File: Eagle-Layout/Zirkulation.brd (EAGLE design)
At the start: 50 x 50 mm, 13 parts, among them X1 MKDSN1,5/3-5,08

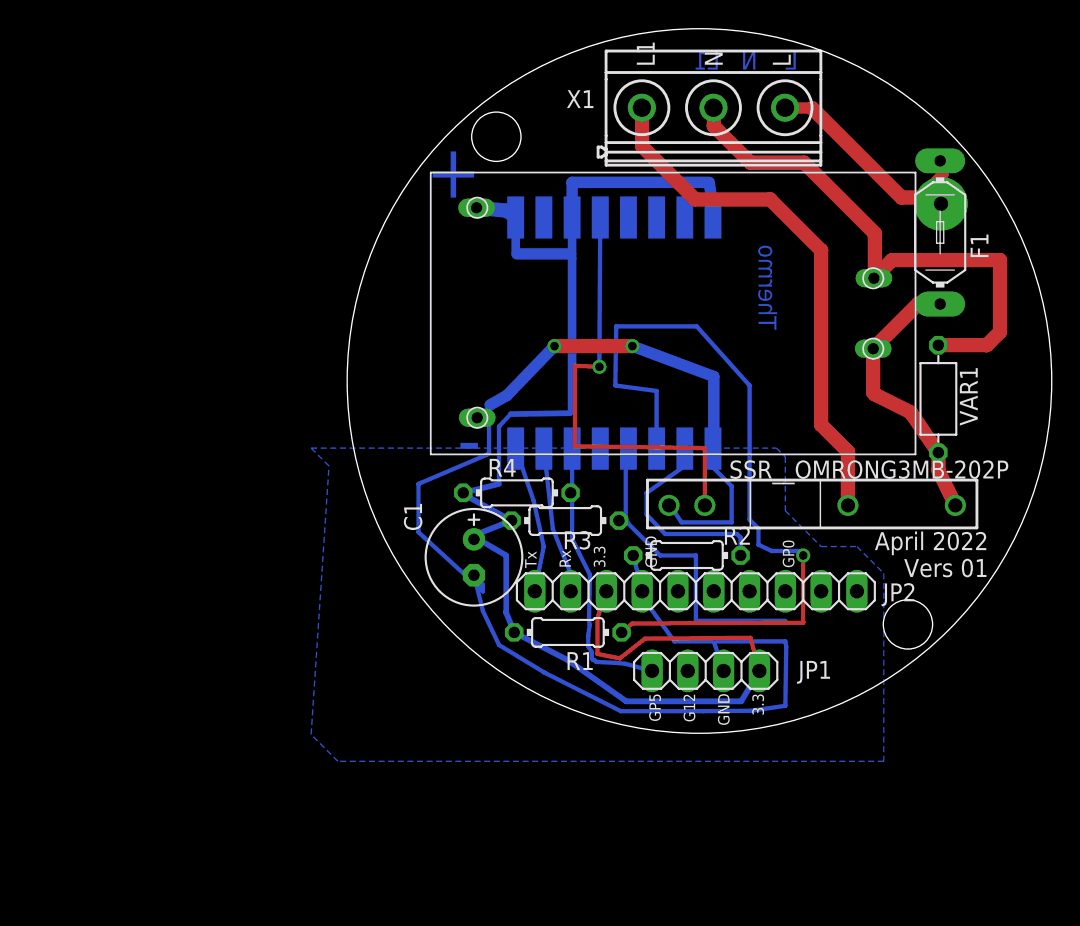
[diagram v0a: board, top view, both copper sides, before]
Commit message: Personal custom variant of Heise Zirkulationspumpe
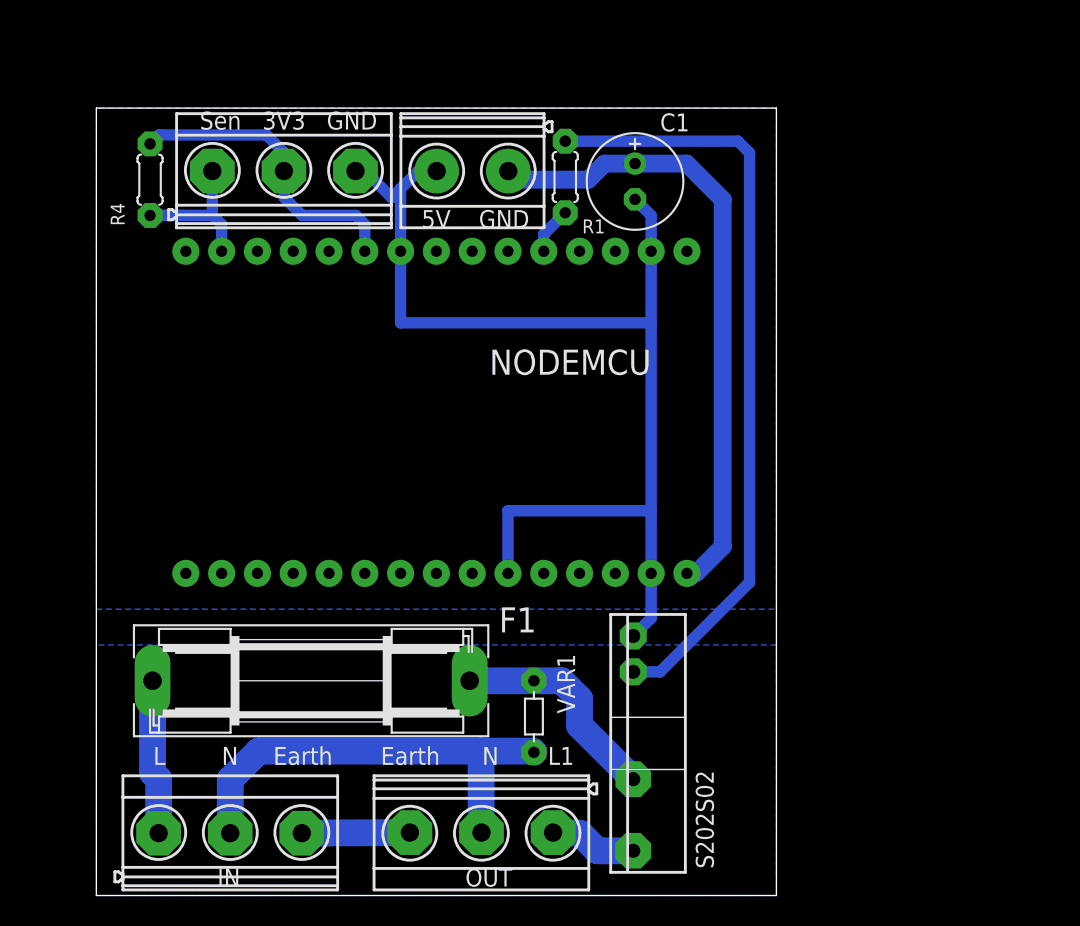
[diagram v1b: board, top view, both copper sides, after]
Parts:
- removed ESP-12E/F: ESP8266, esp8266modules:ESP12-SMD
- removed JP1: Temp.Sensor 18B20, pinhead:1X04
- removed JP2: Prog-Schnittstelle, pinhead:1X10
- removed PRINTTRAFO3.3V,_3W: PRINTTRAFO, Uwes_lib:PRINTTRAFO
- removed R2: 2,2K, rcl:0204/7
- removed R3: 10K, rcl:0204/7
- removed SSR__OMRONG3MB-202P: S102S02, relay:S202S02
- removed X1: MKDSN1,5/3-5,08, con-phoenix-508:MKDSN1,5/3-5,08
- added IN, OUT, SENSOR: MKDSN1,5/3-5,08, my_con-phoenix-508:MKDSN1,5/3-5,08
- added NODEMCU: ESP12E_DEVKIT, ESP12E_DEVKIT:ESP12E_DEVKIT
- added PWR: MKDSN1,5/2-5,08, my_con-phoenix-508:MKDSN1,5/2-5,08
- added S202S02: S202S02, my_relay:S202S02
- C1: device rcl:E2,5-7 -> my_rcl:E2,5-7
- F1: value 1,5A -> 1A; device fuse:LITTLEFUSE -> my_fuse:SH22,5
- R1: device rcl:0204/7 -> my_rcl:0204/5
- R4: value 10K -> 4K7; device rcl:0204/7 -> my_rcl:0204/5
- VAR1: value VARISTOR-7,5 -> VARISTOR-5; device varistor:R-7,5 -> my_varistor:R-5
- moved F1 54.8 mm to (15.2, 15.2), turned to 0 degrees
- moved VAR1 36.5 mm to (31.1, 12.7), turned to 270 degrees
- moved R4 34.2 mm to (3.81, 50.8), turned to 90 degrees
- moved R1 32.3 mm to (33.3, 51.0), turned to 90 degrees
- moved C1 29.0 mm to (38.2, 50.7)
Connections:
- removed net 3.3V: C1.+, ESP-12E/F.CH_PD, ESP-12E/F.RESET, ESP-12E/F.VCC, JP1.1, JP2.3, PRINTTRAFO3.3V,_3W.+, R1.2, R3.2, R4.2
- removed net GPIO0: ESP-12E/F.GPIO0, R3.1
- removed net GPIO15: ESP-12E/F.GPIO15, R2.2
- removed net GPIO16: ESP-12E/F.GPIO16, SSR__OMRONG3MB-202P.3
- removed net GPIO2: ESP-12E/F.GPIO2, R1.1
- removed net GPIO5: ESP-12E/F.GPIO4, JP1.4, R4.1
- removed net L_: F1.2, PRINTTRAFO3.3V,_3W.AC, SSR__OMRONG3MB-202P.1, VAR1.1
- removed net RX: ESP-12E/F.RXD0, JP2.2
- removed net TX: ESP-12E/F.TXD0, JP2.1
- new net G: IN.3, OUT.3
- new net LF: F1.2, S202S02.2, VAR1.1
- new net N$2: R1.2, S202S02.3
- new net N$5: NODEMCU.D8, R1.1
- new net N$6: NODEMCU.3V3@1, R4.2, SENSOR.2
- new net N$7: NODEMCU.D1, R4.1, SENSOR.1
- new net VCC: C1.+, NODEMCU.VIN, PWR.1
- net GND: now also NODEMCU.GND@0, NODEMCU.GND@1, NODEMCU.GND@2, NODEMCU.GND@3, PWR.2, S202S02.4, SENSOR.3; no longer ESP-12E/F.GND, JP1.2, JP2.4, PRINTTRAFO3.3V,_3W.-, R2.1, SSR__OMRONG3MB-202P.4
- net L: now also IN.1; no longer X1.3
- net L1: now also OUT.1, S202S02.1; no longer SSR__OMRONG3MB-202P.2, X1.1
- net N: now also IN.2, OUT.2; no longer PRINTTRAFO3.3V,_3W.~, X1.2
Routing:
- net 3.3V: track 104.9 -> 0.00 mm
- net GPIO2: track 55.4 -> 0.00 mm, vias 1 -> 0
- net N$2: track 0.00 -> 54.8 mm
- net VCC: track 0.00 -> 45.0 mm
- net GPIO16: track 31.3 -> 0.00 mm, vias 1 -> 0
- net L1: track 37.4 -> 6.21 mm
- net GPIO0: track 22.6 -> 0.00 mm
- net GND: track 103.5 -> 81.2 mm, vias 2 -> 0
- net N$6: track 0.00 -> 21.9 mm
- net GPIO5: track 19.8 -> 0.00 mm
- net L_: track 19.7 -> 0.00 mm
- net GPIO15: track 17.7 -> 0.00 mm
- net LF: track 0.00 -> 15.6 mm
- net N$7: track 0.00 -> 12.9 mm
- net TX: track 10.5 -> 0.00 mm
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- added copper zone on layer 16, net COPPER
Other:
- board size 50 x 50 mm -> 48.3 x 55.9 mm
- board text added: "5V GND"
- board text added: "Earth N L1"
- board text added: "L N Earth"
- board text added: "Sen 3V3 GND"
- board text removed: "+"
- board text removed: "-"
- board text removed: "April 2022 Vers 01"
- board text removed: "GP5 G12 GND 3.3"
- board text removed: "L N L1"
- board text removed: "L1 N L"
- board text removed: "Thermo"
- board text removed: "Tx Rx 3.3 GND GP0"
